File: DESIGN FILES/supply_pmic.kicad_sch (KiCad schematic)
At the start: 32 parts, among them U5 UM805RE, U6 UM803RS

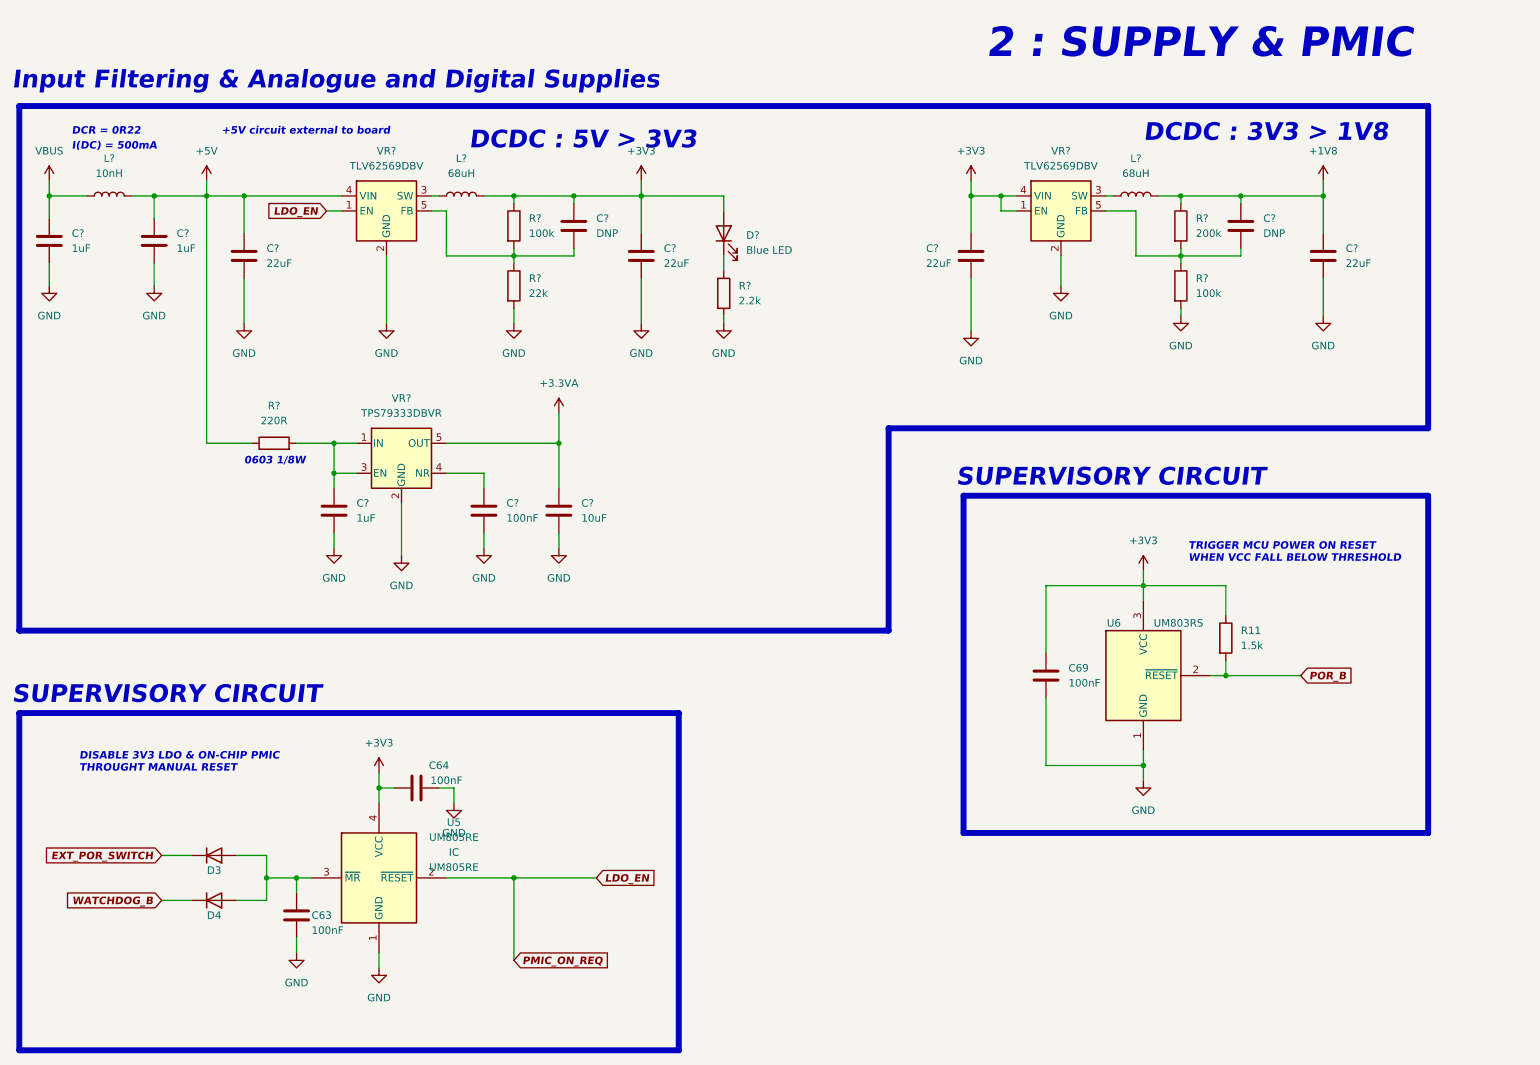
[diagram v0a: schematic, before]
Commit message: schematic edit
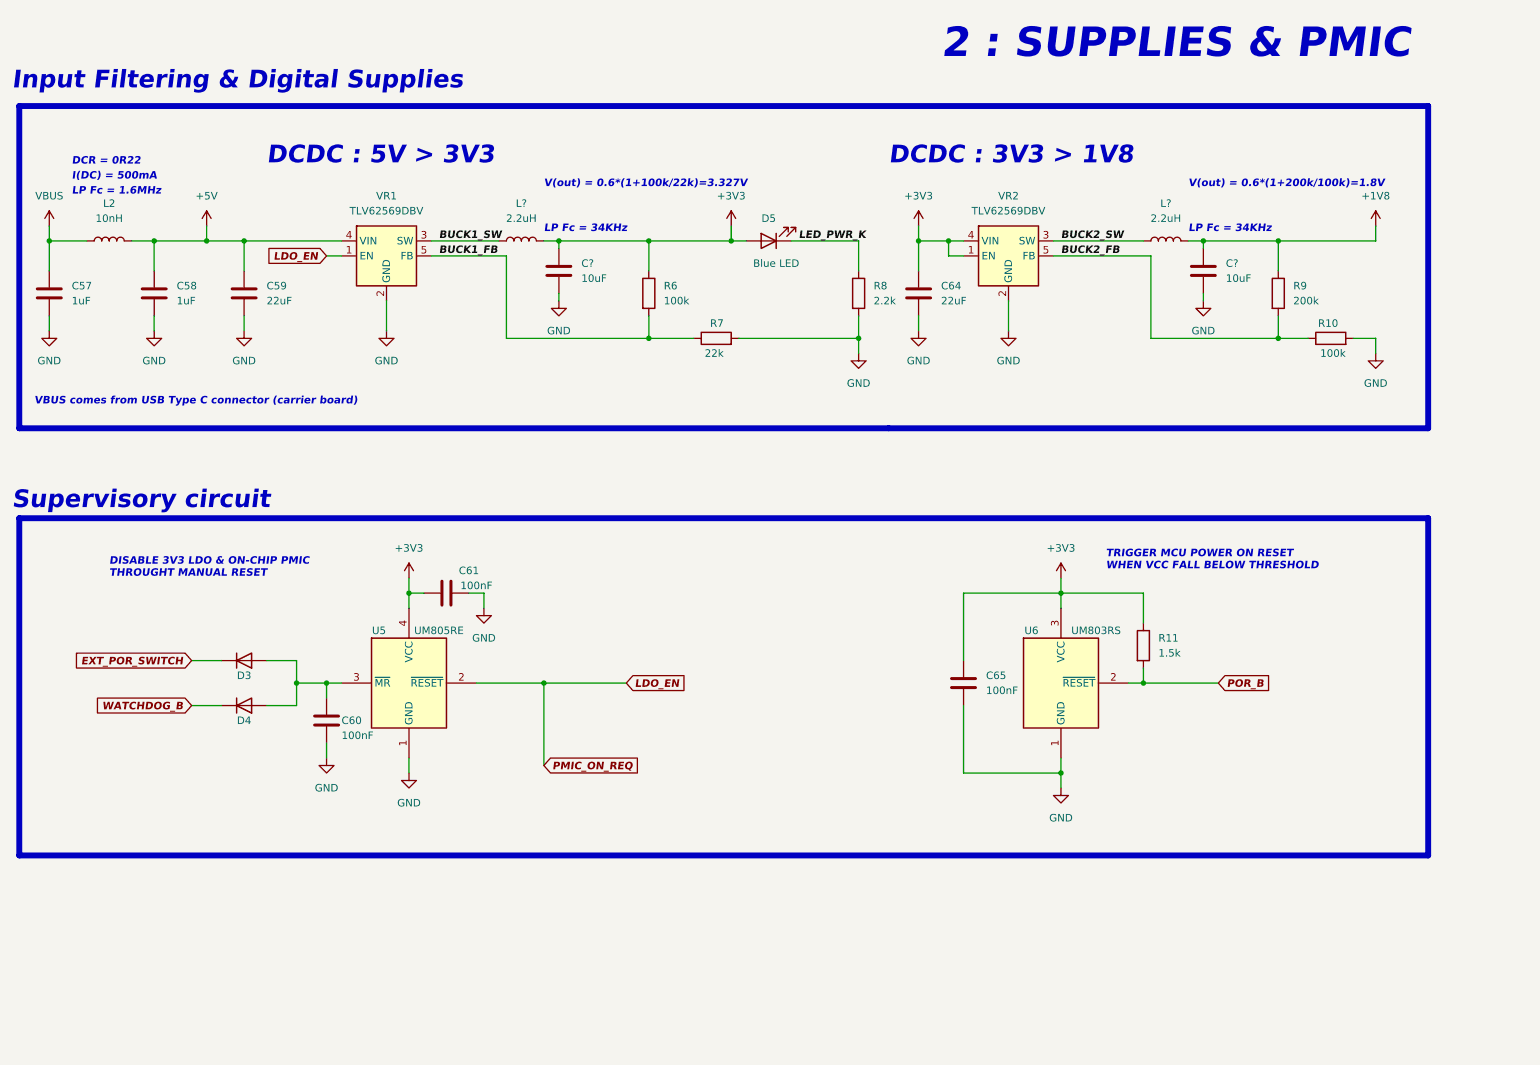
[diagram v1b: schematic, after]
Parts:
- removed C?: 100nF, symbol MIMXRT1064 MCU Module:CL05B104KB54PNC
- removed C?: 1uF, symbol MIMXRT1064 MCU Module:CL05A105KA5NQNC
- removed C? (x2): DNP, MIMXRT1064 MCU Module:0603_CL10A226MQ8NRNC, symbol MIMXRT1064 MCU Module:CL10A226MQ8NRNC
- removed C? (x2): 22uF, MIMXRT1064 MCU Module:0603_CL10A226MQ8NRNC, symbol MIMXRT1064 MCU Module:CL10A226MQ8NRNC
- removed C?: 10uF, symbol MIMXRT1064 MCU Module:CL10A106KP8NNNC
- removed L? (x2): 68uH, symbol MIMXRT1064 MCU Module:MPIT4030-680M-LF
- removed R?: 220R, symbol MIMXRT1064 MCU Module:0603WAF2200T5E
- removed VR?: TPS79333DBVR, Package_TO_SOT_SMD:SOT-23-5, symbol MIMXRT1064 MCU Module:TPS79333DBVR
- added C? (x2): 10uF, symbol MIMXRT1064 MCU Module:CL10A106KP8NNNC
- added L? (x2): 2.2uH, symbol MIMXRT1064 MCU Module:CD32YP0302-2R2M
- C57, C58: renamed from C?; footprint (none) -> MIMXRT1064 MCU Module:0402_CL05A105KA5NQNC
- D5: renamed from D?; footprint (none) -> MIMXRT1064 MCU Module:19-218_BHC-ZL1M2QY_3T
- gave numbers to parts that had none: 10
- renumbered C63 to C60, C64 to C61, C69 to C65
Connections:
- net +1V8: now also C?.1, L?.2
- net +3V3: now also C?.1, L?.2
- net GND: now also C?.2, C?.2
- net LED_PWR_K: now reaches D5.1 (K), R8.1
- net BUCK2_SW: now reaches VR2.3 (SW)
- net BUCK2_SW: now also L?.1
- net BUCK2_FB: now reaches R10.1, R9.2, VR2.5 (FB)
- net BUCK1_FB: now reaches R6.2, R7.1, VR1.5 (FB)
- net BUCK1_SW: now reaches VR1.3 (SW)
- net BUCK1_SW: now also L?.1
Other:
- note added: "2 : SUPPLIES & PMIC"
- note added: "Input Filtering & Digital Supplies"
- note added: "LP Fc = 1.6MHz"
- note added: "LP Fc = 34KHz"
- note added: "Supervisory circuit"
- note added: "V(out) = 0.6*(1+100k/22k)=3.327V"
- note added: "V(out) = 0.6*(1+200k/100k)=1.8V"
- note added: "VBUS comes from USB Type C connector (carrier board)"
- note removed: "+5V circuit external to board"
- note removed: "0603 1/8W"
- note removed: "2 : SUPPLY & PMIC"
- note removed: "Input Filtering & Analogue and Digital Supplies"
- note removed: "SUPERVISORY CIRCUIT"
- moved on the sheet: C57, C58, C59, C60, C61, C64, C65, D3, D4, D5, L2, R10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
